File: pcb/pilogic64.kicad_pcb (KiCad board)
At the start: 2 copper layers, 8 parts, among them SW1 RotaryEncoder_Switch, SW2 RotaryEncoder_Switch, U2 Pico

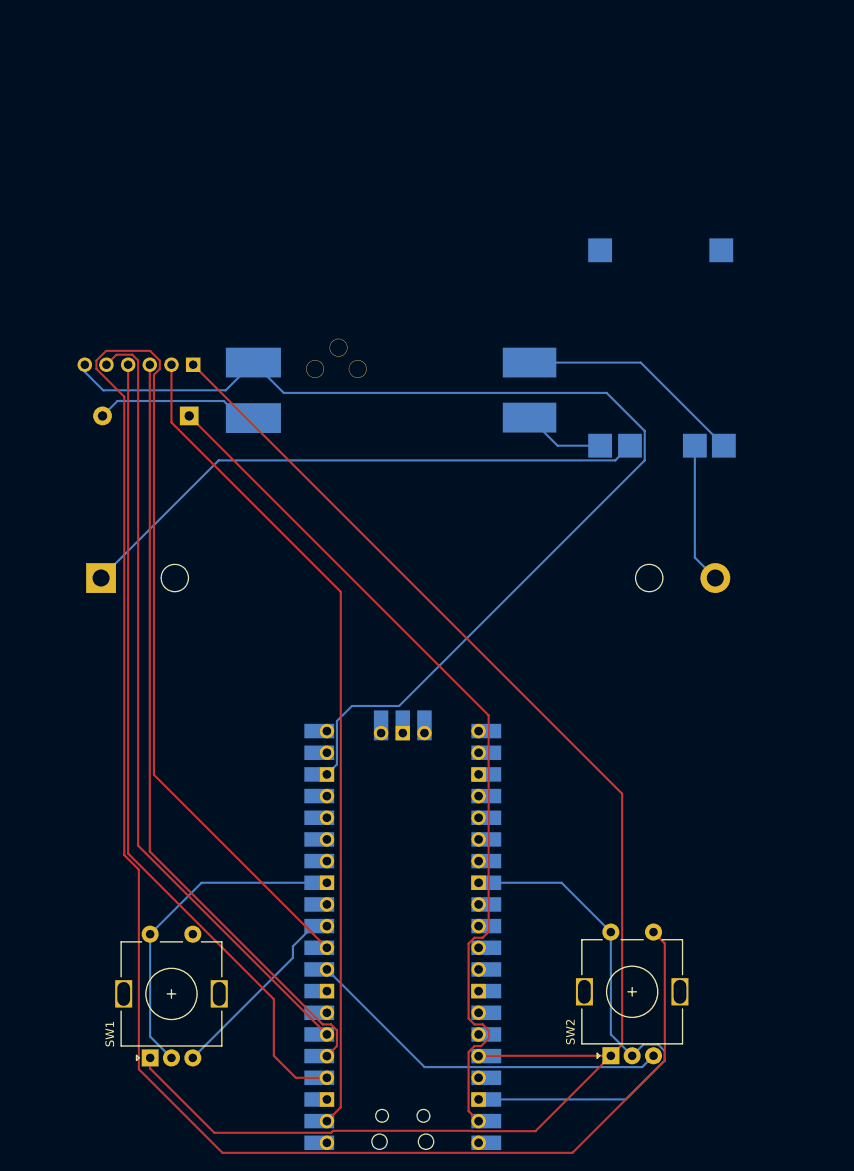
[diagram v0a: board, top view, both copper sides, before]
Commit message: Finished cicuit, and I think also finished pcb
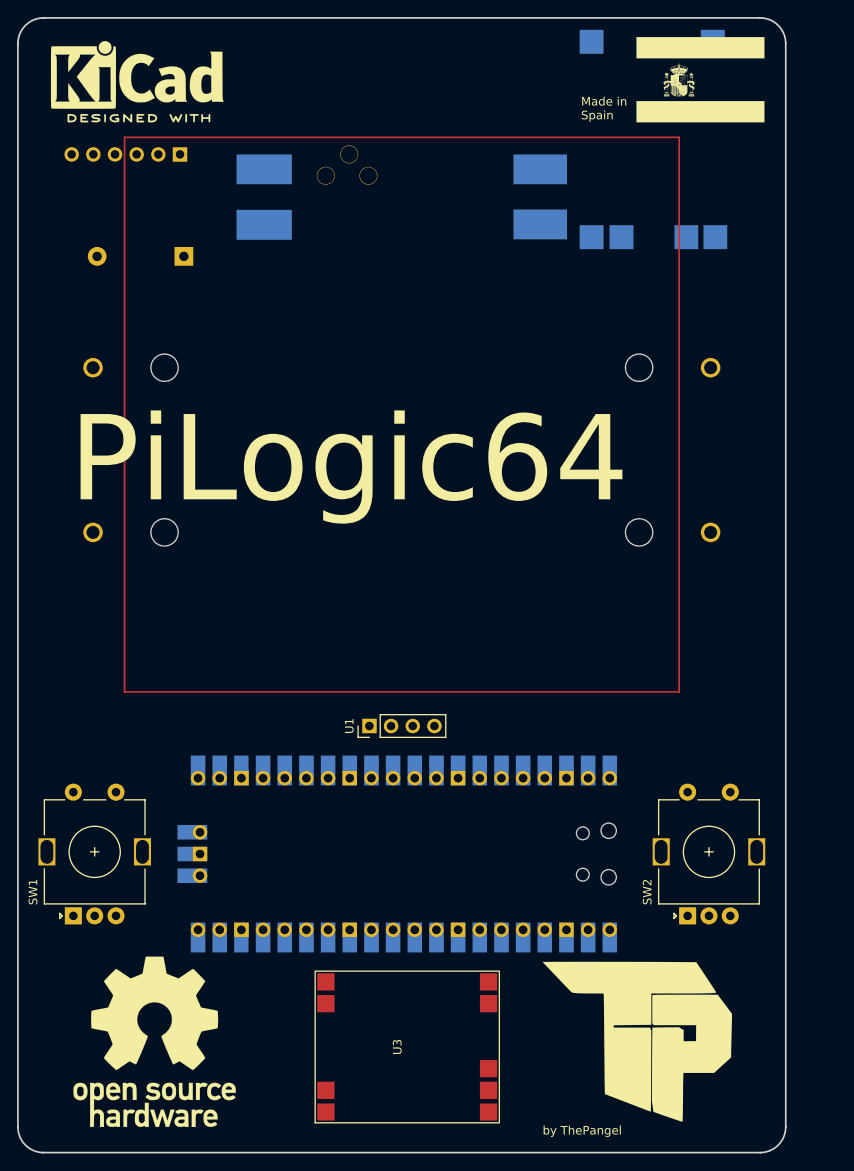
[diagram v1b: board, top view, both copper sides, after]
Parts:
- added G***: LOGO, LOGO, F.Cu at (178.0, 36.6)
- added G***: LOGO, LOGO, F.Cu at (171.0, 149.3)
- added REF**: KiCad-Logo2_8mm_SilkScreen, Symbol:KiCad-Logo2_8mm_SilkScreen, F.Cu at (112.0, 36.0)
- added REF**: OSHW-Logo_19x20mm_SilkScreen, Symbol:OSHW-Logo_19x20mm_SilkScreen, F.Cu at (114.0, 149.3)
- added U1: ~, Connector_PinHeader_2.54mm:PinHeader_1x04_P2.54mm_Vertical, F.Cu at (139.2, 112.3)
- added U3: pam8403, Library:pam8403, F.Cu at (143.0, 150.0)
- b18650: footprint Battery:BatteryHolder_MPD_BH-18650-PC2 -> Library:18650-PC4
- moved b18650 38.3 mm to (143.0, 80.0)
- moved SD_SPI1 24.7 mm to (117.0, 45.3)
- moved TP4056-18650 24.5 mm to (163.5, 30.4)
- moved MT3608_module_SMT1 22.7 mm to (144.6, 50.3)
- moved SW1 18.9 mm to (104.5, 134.6)
- moved D1 18.7 mm to (117.5, 57.3)
- moved SW2 18.7 mm to (176.5, 134.6)
- moved U2 9.72 mm to (143.2, 127.3), turned to 90 degrees
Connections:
- U2 pad 14: unconnected-(U2-GPIO10-Pad14) -> Net-(U1-SDA)
- U2 pad 15: unconnected-(U2-GPIO11-Pad15) -> Net-(U1-SCL)
- U2 pad 19: unconnected-(U2-GPIO14-Pad19) -> Net-(U2-GPIO14)
- U2 pad 20: unconnected-(U2-GPIO15-Pad20) -> Net-(U2-GPIO15)
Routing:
- net Net-(U2-GPIO7): track 256.8 -> 0.00 mm
- net GND: track 232.8 -> 0.00 mm
- net +3.3V: track 180.0 -> 0.00 mm
- net Net-(D1-K): track 102.2 -> 0.00 mm
- net Net-(SD_SPI1-cs): track 97.6 -> 0.00 mm
- net Net-(SD_SPI1-CLK): track 95.4 -> 0.00 mm
- net Net-(SD_SPI1-MISO): track 92.6 -> 0.00 mm
- net Net-(SD_SPI1-MOSI): track 91.2 -> 0.00 mm
- net Net-(TP4056-18650-B+): track 68.4 -> 0.00 mm
- net Net-(U2-GPIO6): track 43.6 -> 0.00 mm
- net Net-(MT3608_module_SMT1-VIN-): track 26.8 -> 0.00 mm
- net Net-(U2-GPIO8): track 22.9 -> 0.00 mm
- net +5V: track 19.2 -> 0.00 mm
- net Net-(TP4056-18650-B-): track 16.5 -> 0.00 mm
- net Net-(MT3608_module_SMT1-VIN+): track 9.63 -> 0.00 mm
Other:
- board outline added: 90 x 133 mm
- board text added: "Made in Spain"
- board text added: "PiLogic64"
- board text added: "by ThePangel"
